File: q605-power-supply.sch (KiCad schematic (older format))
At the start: 18 parts, among them J1 ATX-24, J2 Screw_Terminal_01x02, J3 Screw_Terminal_01x02, J4 Screw_Terminal_01x05, J5 Conn_01x06, Q1 Q_NPN_CBE, U1 PIC16F18313, U2 MC79M05_TO220

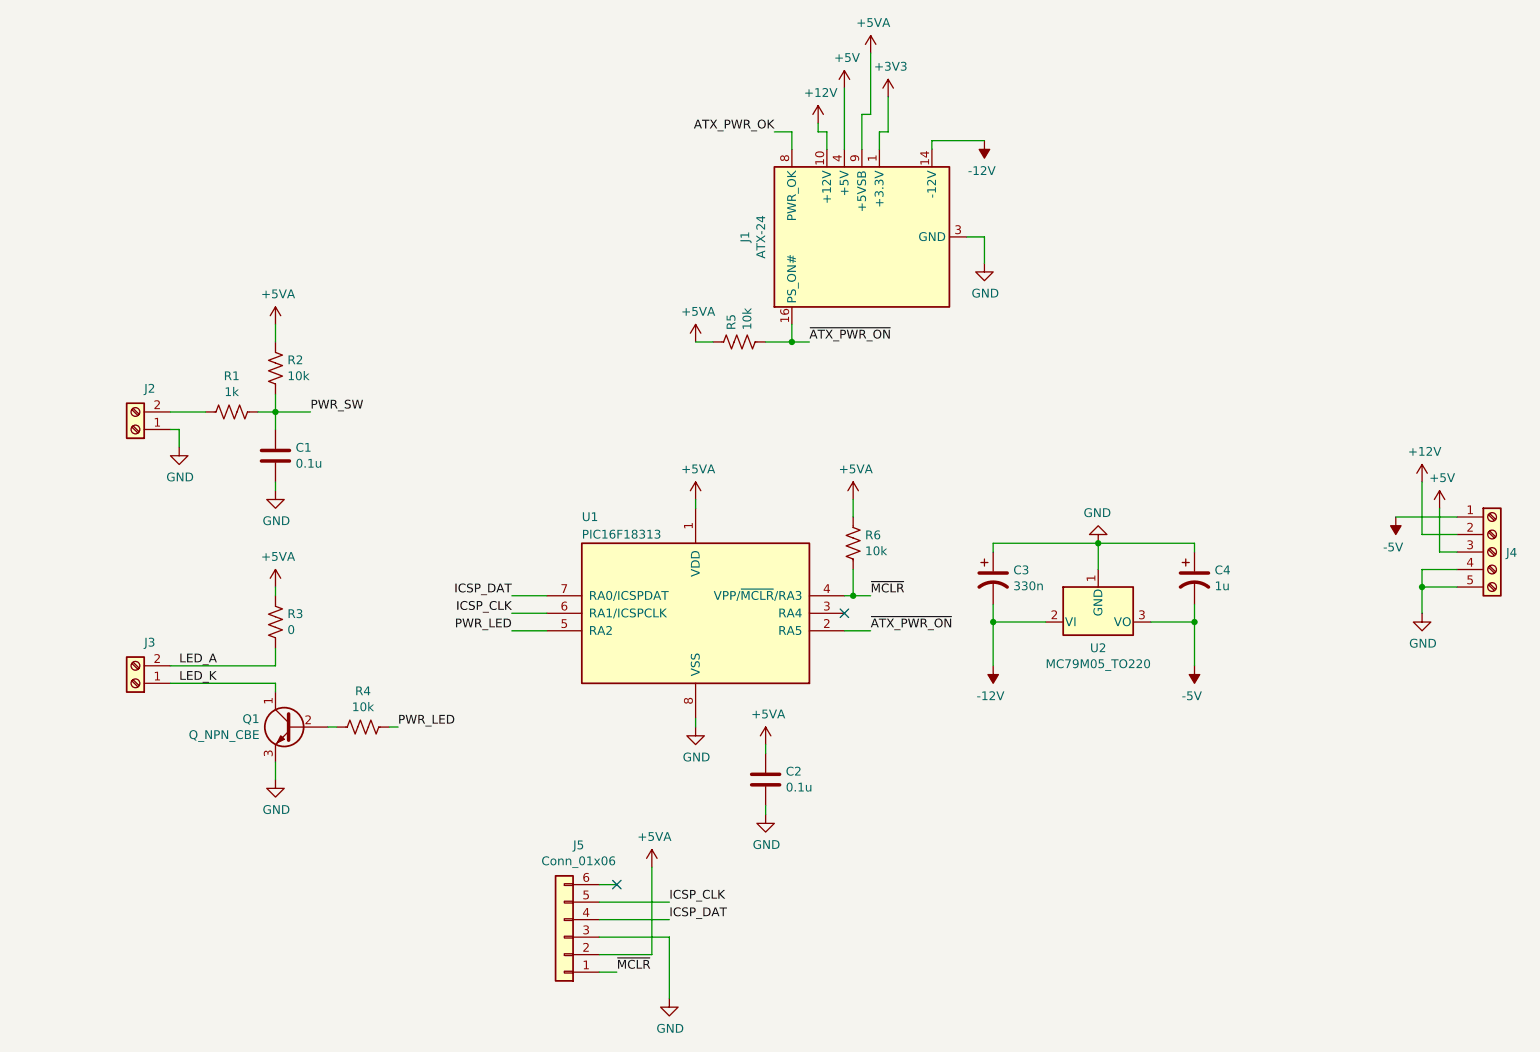
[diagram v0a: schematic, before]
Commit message: Finished routing
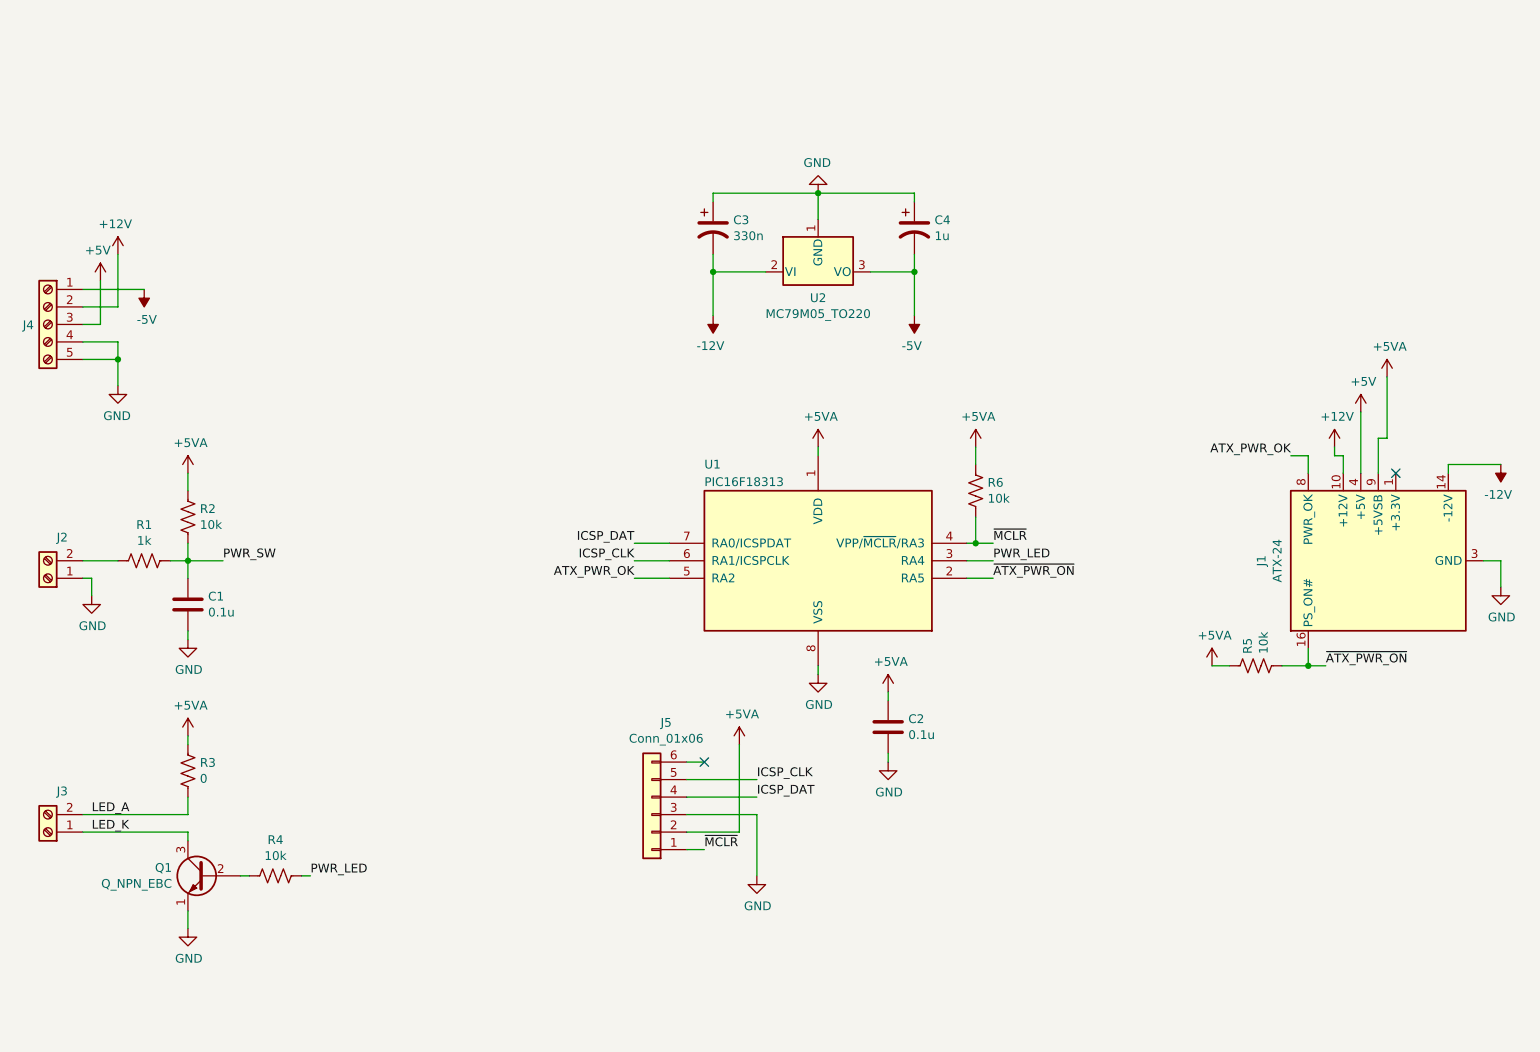
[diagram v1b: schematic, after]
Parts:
- removed Q1: Q_NPN_CBE, Package_TO_SOT_THT:TO-92, symbol Device:Q_NPN_CBE
- added Q1: Q_NPN_EBC, Package_TO_SOT_THT:TO-92, symbol Device:Q_NPN_EBC
- J2, J3: footprint TerminalBlock_TE-Connectivity:TerminalBlock_TE_282834-2_1x02_P2.54mm_Horizontal -> TerminalBlock_RND:TerminalBlock_RND_205-00001_1x02_P5.00mm_Horizontal
- J4: footprint TerminalBlock_TE-Connectivity:TerminalBlock_TE_282834-5_1x05_P2.54mm_Horizontal -> TerminalBlock_RND:TerminalBlock_RND_205-00004_1x05_P5.00mm_Horizontal
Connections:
- net ATX_PWR_OK: now also U1.5 (RA2)
- net GND: now also Q1.1 (E)
- net LED_K: now also Q1.3 (C)
- net PWR_LED: now also U1.3 (RA4); no longer U1.5 (RA2)
- net at R4.2: now also Q1.2 (B)
- net +3V3: no longer names the net of J1.1 (+3.3V), J1.12 (+3.3V), J1.13 (+3.3V), J1.2 (+3.3V)
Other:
- moved on the sheet: C1, C2, C3, C4, J1, J2, J3, J4, J5, R1, R2, R3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
